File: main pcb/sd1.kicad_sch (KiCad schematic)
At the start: 14 parts

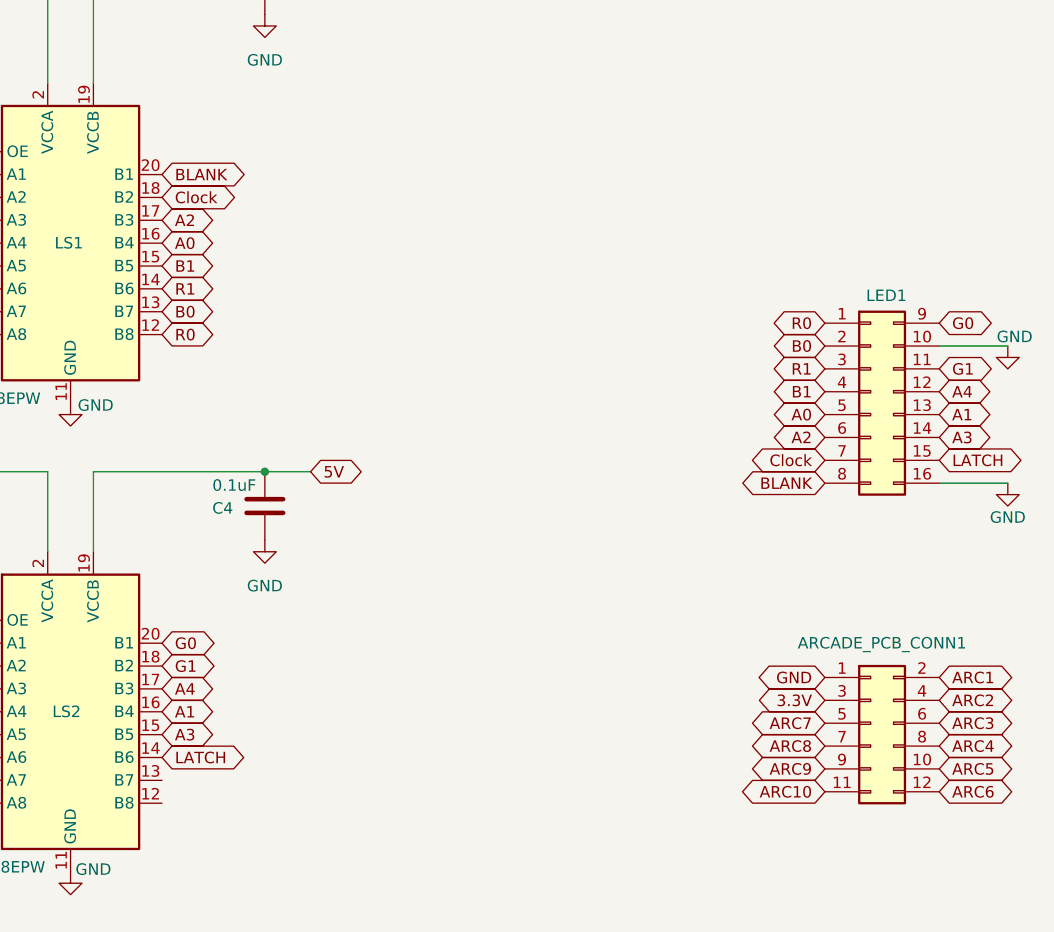
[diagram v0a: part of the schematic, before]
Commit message: update main pcb
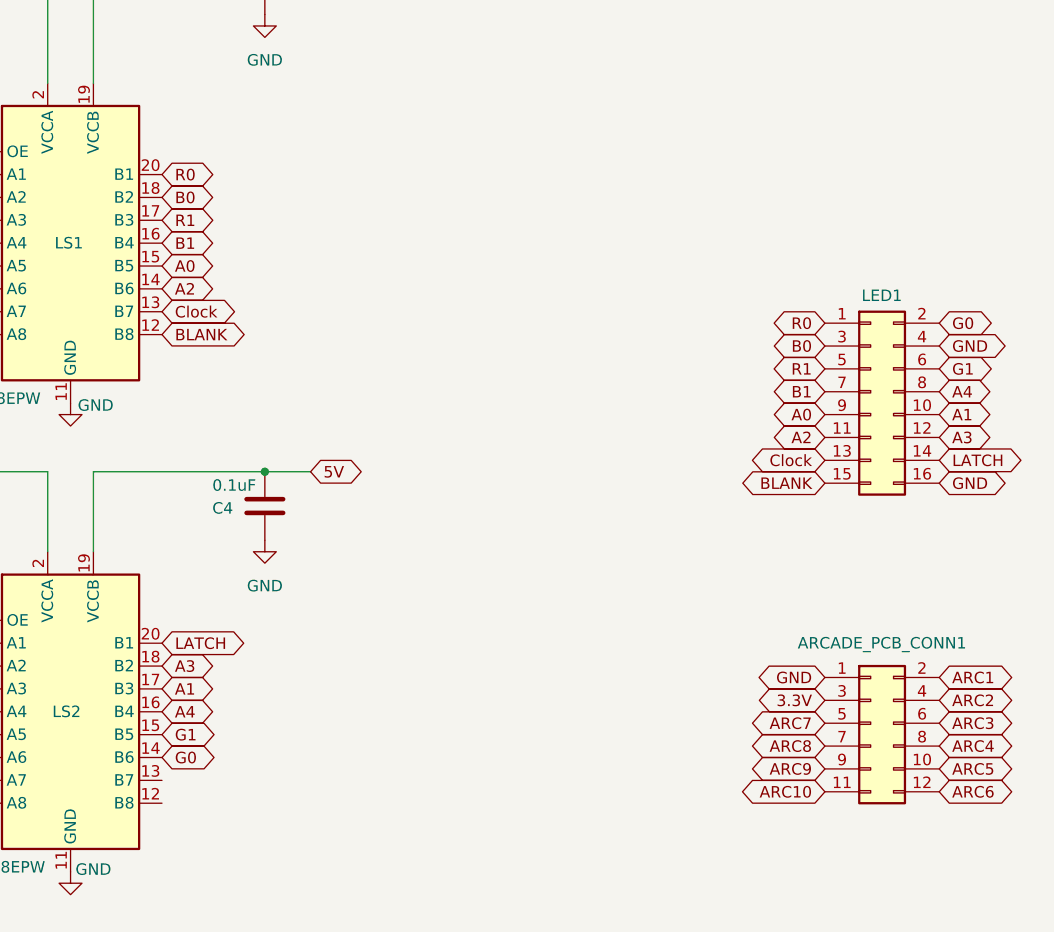
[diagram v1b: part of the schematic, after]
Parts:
- LED1: value Conn_02x08_Top_Bottom -> Conn_02x08_Odd_Even; symbol Connector_Generic:Conn_02x08_Top_Bottom -> Connector_Generic:Conn_02x08_Odd_Even
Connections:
- net A0: now also LED1.9 (Pin_9), LS1.15 (B5); no longer LED1.5 (Pin_5), LS1.16 (B4)
- net A1: now also LED1.10 (Pin_10), LS2.17 (B3); no longer LED1.13 (Pin_13), LS2.16 (B4)
- net A2: now also LED1.11 (Pin_11), LS1.14 (B6); no longer LED1.6 (Pin_6), LS1.17 (B3)
- net A3: now also LED1.12 (Pin_12), LS2.18 (B2); no longer LED1.14 (Pin_14), LS2.15 (B5)
- net A4: now also LED1.8 (Pin_8), LS2.16 (B4); no longer LED1.12 (Pin_12), LS2.17 (B3)
- net B0: now also LED1.3 (Pin_3), LS1.18 (B2); no longer LED1.2 (Pin_2), LS1.13 (B7)
- net B1: now also LED1.7 (Pin_7), LS1.16 (B4); no longer LED1.4 (Pin_4), LS1.15 (B5)
- net BLANK: now also LED1.15 (Pin_15), LS1.12 (B8); no longer LED1.8 (Pin_8), LS1.20 (B1)
- net Clock: now also LED1.13 (Pin_13), LS1.13 (B7); no longer LED1.7 (Pin_7), LS1.18 (B2)
- net G0: now also LED1.2 (Pin_2), LS2.14 (B6); no longer LED1.9 (Pin_9), LS2.20 (B1)
- net G1: now also LED1.6 (Pin_6), LS2.15 (B5); no longer LED1.11 (Pin_11), LS2.18 (B2)
- net GND: now also LED1.4 (Pin_4); no longer LED1.10 (Pin_10)
- net LATCH: now also LED1.14 (Pin_14), LS2.20 (B1); no longer LED1.15 (Pin_15), LS2.14 (B6)
- net R0: now also LS1.20 (B1); no longer LS1.12 (B8)
- net R1: now also LED1.5 (Pin_5), LS1.17 (B3); no longer LED1.3 (Pin_3), LS1.14 (B6)
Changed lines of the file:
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@@
 		)
 	)
-	(wire
-		(pts
-			(xy 266.7 82.55) (xy 274.32 82.55)
-		)
-		(stroke
-			(width 0)
-			(type default)
-		)
-	)
 	(polyline
 		(pts
@@
 	(wire
 		(pts
-			(xy 266.7 97.79) (xy 274.32 97.79)
-		)
-		(stroke
-			(width 0)
-			(type default)
-		)
-	)
-	(wire
-		(pts
 			(xy 50.8 67.31) (xy 50.8 69.85)
 		)
@@
 	(global_label "A0"
 		(shape bidirectional)
-		(at 180.34 71.12 0)
+		(at 180.34 73.66 0)
 		(fields_autoplaced yes)
 		(effects
@@
 		)
 		(property "Intersheetrefs" "${INTERSHEET_REFS}"
-			(at 186.7346 71.12 0)
+			(at 186.7346 73.66 0)
 			(effects
 				(font
@@
 	(global_label "B1"
 		(shape bidirectional)
-		(at 180.34 73.66 0)
+		(at 180.34 71.12 0)
 		(fields_autoplaced yes)
 		(effects
@@
 		)
 		(property "Intersheetrefs" "${INTERSHEET_REFS}"
-			(at 186.916 73.66 0)
+			(at 186.916 71.12 0)
 			(effects
 				(font
@@
 	(global_label "A4"
 		(shape bidirectional)
-		(at 180.34 120.65 0)
+		(at 180.34 123.19 0)
 		(fields_autoplaced yes)
 		(effects
@@
 		)
 		(property "Intersheetrefs" "${INTERSHEET_REFS}"
-			(at 186.7346 120.65 0)
+			(at 186.7346 123.19 0)
 			(effects
 				(font
@@
 		)
 	)
+	(global_label "GND"
+		(shape bidirectional)
+		(at 266.7 82.55 0)
+		(fields_autoplaced yes)
+		(effects
+			(font
+				(size 1.27 1.27)
+			)
+			(justify left)
+		)
+		(property "Intersheetrefs" "${INTERSHEET_REFS}"
+			(at 274.667 82.55 0)
+			(effects
+				(font
+					(size 1.27 1.27)
+				)
+				(justify left)
+				(hide yes)
+			)
+		)
+	)
 	(global_label "ARC10"
 		(shape bidirectional)
@@
 	(global_label "R1"
 		(shape bidirectional)
-		(at 180.34 76.2 0)
+		(at 180.34 68.58 0)
 		(fields_autoplaced yes)
 		(effects
@@
 		)
 		(property "Intersheetrefs" "${INTERSHEET_REFS}"
-			(at 186.916 76.2 0)
+			(at 186.916 68.58 0)
 			(effects
 				(font
@@
 	(global_label "R0"
 		(shape bidirectional)
-		(at 180.34 81.28 0)
+		(at 180.34 63.5 0)
 		(fields_autoplaced yes)
 		(effects
@@
 		)
 		(property "Intersheetrefs" "${INTERSHEET_REFS}"
-			(at 186.916 81.28 0)
+			(at 186.916 63.5 0)
 			(effects
 				(font
@@
 	(global_label "LATCH"
 		(shape bidirectional)
-		(at 180.34 128.27 0)
+		(at 180.34 115.57 0)
 		(fields_autoplaced yes)
 		(effects
@@
 		)
 		(property "Intersheetrefs" "${INTERSHEET_REFS}"
-			(at 190.1213 128.27 0)
+			(at 190.1213 115.57 0)
 			(effects
 				(font
@@
 	(global_label "G0"
 		(shape bidirectional)
-		(at 180.34 115.57 0)
+		(at 180.34 128.27 0)
 		(fields_autoplaced yes)
 		(effects
@@
 		)
 		(property "Intersheetrefs" "${INTERSHEET_REFS}"
-			(at 186.916 115.57 0)
+			(at 186.916 128.27 0)
 			(effects
 				(font
@@
 	(global_label "B0"
 		(shape bidirectional)
-		(at 180.34 78.74 0)
+		(at 180.34 66.04 0)
 		(fields_autoplaced yes)
 		(effects
@@
 		)
 		(property "Intersheetrefs" "${INTERSHEET_REFS}"
-			(at 186.916 78.74 0)
+			(at 186.916 66.04 0)
+			(effects
+				(font
+					(size 1.27 1.27)
+				)
+				(justify left)
+				(hide yes)
+			)
+		)
+	)
+	(global_label "GND"
+		(shape bidirectional)
+		(at 266.7 97.79 0)
+		(fields_autoplaced yes)
+		(effects
+			(font
+				(size 1.27 1.27)
+			)
+			(justify left)
+		)
+		(property "Intersheetrefs" "${INTERSHEET_REFS}"
+			(at 274.667 97.79 0)
 			(effects
 				(font
@@
 	(global_label "A1"
 		(shape bidirectional)
-		(at 180.34 123.19 0)
+		(at 180.34 120.65 0)
 		(fields_autoplaced yes)
 		(effects
@@
 		)
 		(property "Intersheetrefs" "${INTERSHEET_REFS}"
-			(at 186.7346 123.19 0)
+			(at 186.7346 120.65 0)
 			(effects
 				(font
@@
 	(global_label "G1"
 		(shape bidirectional)
-		(at 180.34 118.11 0)
+		(at 180.34 125.73 0)
 		(fields_autoplaced yes)
 		(effects
@@
 		)
 		(property "Intersheetrefs" "${INTERSHEET_REFS}"
-			(at 186.916 118.11 0)
+			(at 186.916 125.73 0)
 			(effects
 				(font
@@
 	(global_label "A2"
 		(shape bidirectional)
-		(at 180.34 68.58 0)
+		(at 180.34 76.2 0)
 		(fields_autoplaced yes)
 		(effects
@@
 		)
 		(property "Intersheetrefs" "${INTERSHEET_REFS}"
-			(at 186.7346 68.58 0)
+			(at 186.7346 76.2 0)
 			(effects
 				(font
@@
 	(global_label "A3"
 		(shape bidirectional)
-		(at 180.34 125.73 0)
+		(at 180.34 118.11 0)
 		(fields_autoplaced yes)
 		(effects
@@
 		)
 		(property "Intersheetrefs" "${INTERSHEET_REFS}"
-			(at 186.7346 125.73 0)
+			(at 186.7346 118.11 0)
 			(effects
 				(font
@@
 	(global_label "BLANK"
 		(shape bidirectional)
-		(at 180.34 63.5 0)
+		(at 180.34 81.28 0)
 		(fields_autoplaced yes)
 		(effects
@@
 		)
 		(property "Intersheetrefs" "${INTERSHEET_REFS}"
-			(at 190.4237 63.5 0)
+			(at 190.4237 81.28 0)
 			(effects
 				(font
@@
 	(global_label "Clock"
 		(shape bidirectional)
-		(at 180.34 66.04 0)
+		(at 180.34 78.74 0)
 		(fields_autoplaced yes)
 		(effects
@@
 		)
 		(property "Intersheetrefs" "${INTERSHEET_REFS}"
-			(at 189.6374 66.04 0)
+			(at 189.6374 78.74 0)
 			(effects
 				(font
@@
 	)
 	(symbol
-		(lib_id "power:GND")
-		(at 274.32 82.55 0)
-		(unit 1)
-		(exclude_from_sim no)
-		(in_bom yes)
-		(on_board yes)
-		(dnp no)
-		(property "Reference" "#PWR012"
-			(at 274.32 88.9 0)
-			(effects
-				(font
-					(size 1.27 1.27)
-				)
-				(hide yes)
-			)
-		)
-		(property "Value" "GND"
-			(at 275.082 81.534 0)
-			(effects
-				(font
-					(size 1.27 1.27)
-				)
-			)
-		)
-		(property "Footprint" ""
-			(at 274.32 82.55 0)
-			(effects
-				(font
-					(size 1.27 1.27)
-				)
-				(hide yes)
-			)
-		)
-		(property "Datasheet" ""
-			(at 274.32 82.55 0)
-			(effects
-				(font
-					(size 1.27 1.27)
-				)
-				(hide yes)
-			)
-		)
-		(property "Description" "Power symbol creates a global label with name \"GND\" , ground"
-			(at 274.32 82.55 0)
-			(effects
-				(font
-					(size 1.27 1.27)
-				)
-				(hide yes)
-			)
-		)
-		(pin "1"
-		)
-		(instances
-			(project ""
-				(path "/a9c4345d-d258-4ab9-942d-412ef1fae7c9"
-					(reference "#PWR012")
-					(unit 1)
-				)
-			)
-		)
-	)
-	(symbol
 		(lib_id "Connector_Generic:ARCADE_PCB_CONN")
 		(at 259.08 124.46 0)
@@
 	)
 	(symbol
-		(lib_id "Connector_Generic:Conn_02x08_Top_Bottom")
+		(lib_id "Connector_Generic:Conn_02x08_Odd_Even")
 		(at 259.08 87.63 0)
 		(unit 1)
@@
 		(dnp no)
 		(property "Reference" "LED1"
-			(at 258.572 76.962 0)
+			(at 258.064 76.962 0)
 			(effects
 				(font
@@
 			)
 		)
-		(property "Value" "Conn_02x08_Top_Bottom"
-			(at 260.35 123.952 90)
+		(property "Value" "Conn_02x08_Odd_Even"
+			(at 260.35 100.33 0)
 			(effects
 				(font
 					(size 1.27 1.27)
 				)
-				(justify left)
 				(hide yes)
 			)
@@
 			)
 		)
-		(property "Description" "Generic connector, double row, 02x08, top/bottom pin numbering scheme (row 1: 1...pins_per_row, row2: pins_per_row+1 ... num_pins), script generated (kicad-library-utils/schlib/autogen/connector/)"
+		(property "Description" "Generic connector, double row, 02x08, odd/even pin numbering scheme (row 1 odd numbers, row 2 even numbers), script generated (kicad-library-utils/schlib/autogen/connector/)"
 			(at 259.08 87.63 0)
 			(effects
@@
 					(unit 1)
 				)
-			)
-		)
-	)
-	(symbol
-		(lib_id "power:GND")
-		(at 274.32 97.79 0)
-		(unit 1)
-		(exclude_from_sim no)
-		(in_bom yes)
-		(on_board yes)
-		(dnp no)
-		(property "Reference" "#PWR013"
-			(at 274.32 104.14 0)
-			(effects
-				(font
-					(size 1.27 1.27)
-				)
-				(hide yes)
-			)
-		)
-		(property "Value" "GND"
-			(at 274.32 101.6 0)
-			(effects
-				(font
-					(size 1.27 1.27)
-				)
-			)
-		)
-		(property "Footprint" ""
-			(at 274.32 97.79 0)
-			(effects
-				(font
-					(size 1.27 1.27)
-				)
-				(hide yes)
-			)
-		)
-		(property "Datasheet" ""
-			(at 274.32 97.79 0)
-			(effects
-				(font
-					(size 1.27 1.27)
-				)
-				(hide yes)
-			)
-		)
-		(property "Description" "Power symbol creates a global label with name \"GND\" , ground"
-			(at 274.32 97.79 0)
-			(effects
-				(font
-					(size 1.27 1.27)
-				)
-				(hide yes)
-			)
-		)
-		(pin "1"
-		)
-		(instances
-			(project ""
-				(path "/a9c4345d-d258-4ab9-942d-412ef1fae7c9"
-					(reference "#PWR013")
-					(unit 1)
-				)
